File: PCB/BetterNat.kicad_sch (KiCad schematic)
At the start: 7 parts, among them J1 Conn_02x20_Odd_Even_Shielded, SW2 1825910-6, SW3 1825910-6, SW4 1825910-6, U1 KY-040

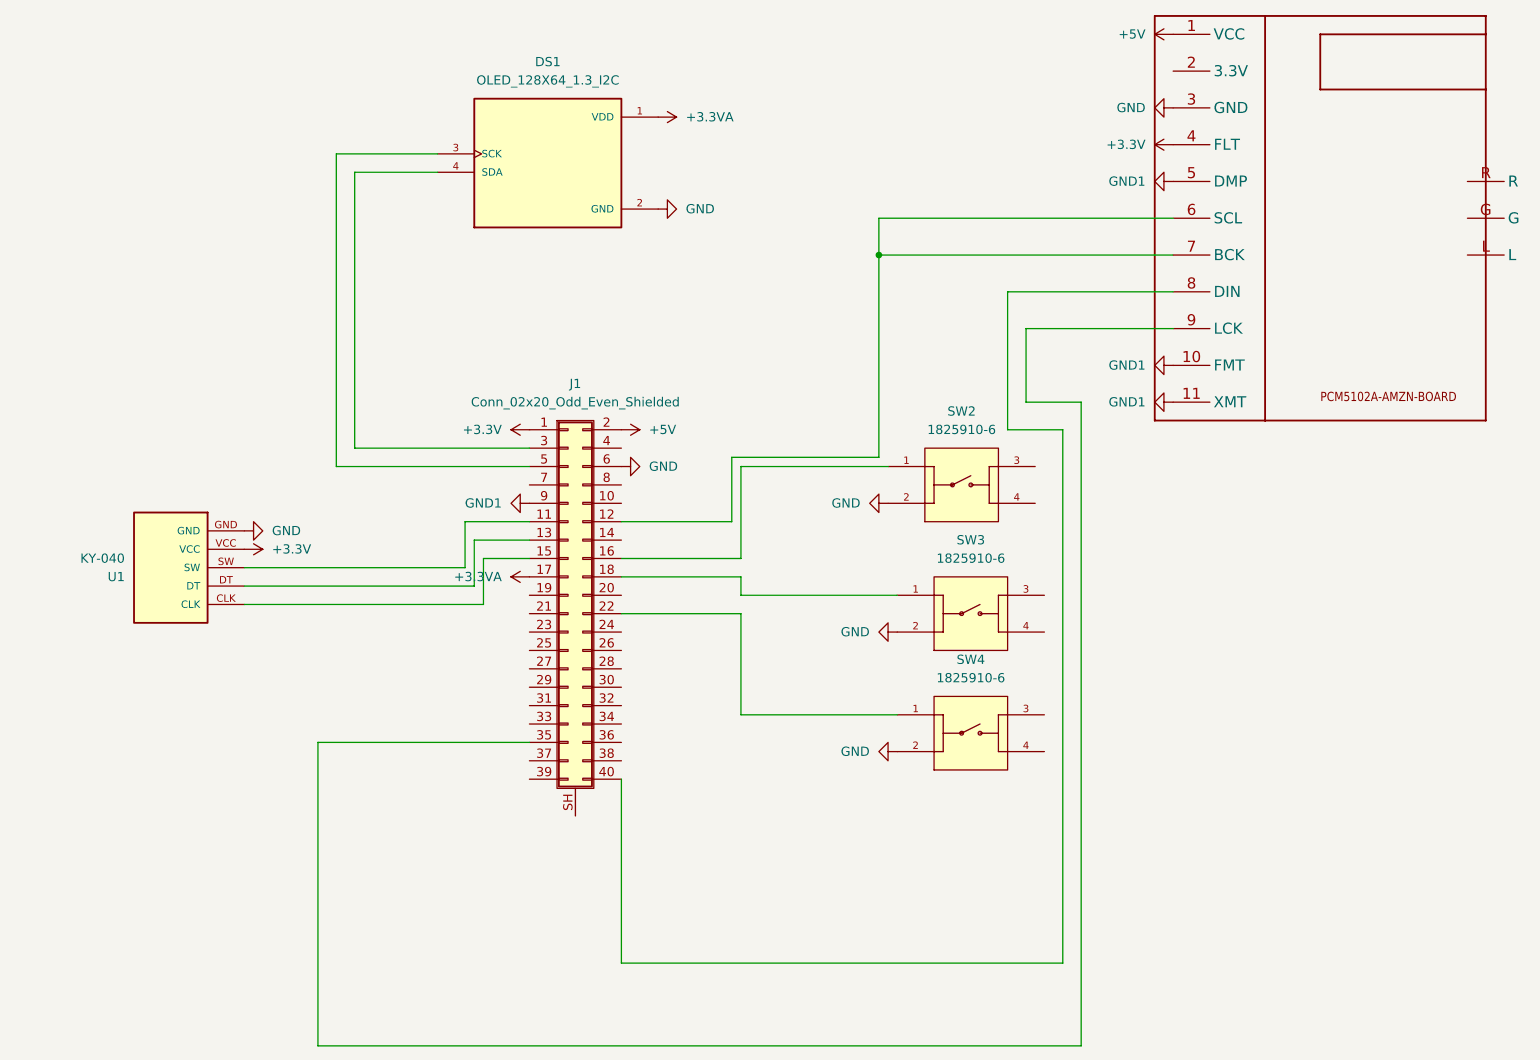
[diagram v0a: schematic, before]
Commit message: update V2
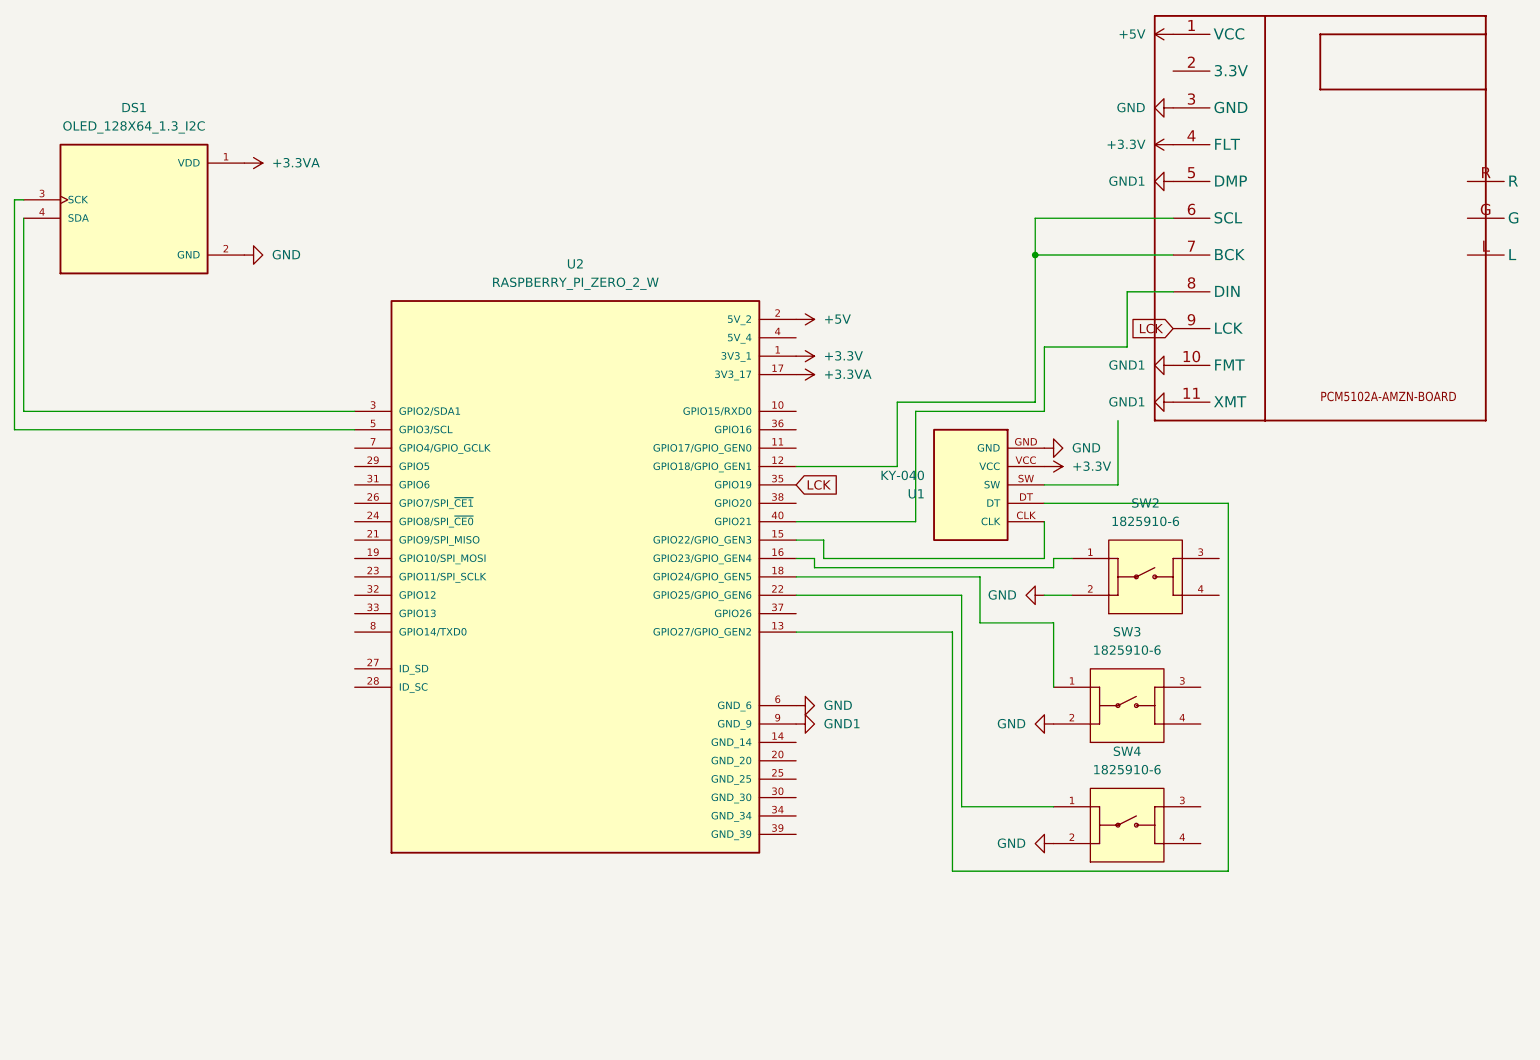
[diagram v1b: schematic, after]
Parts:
- removed J1: Conn_02x20_Odd_Even_Shielded, pin:Pin_Header_Angled_2x20_Pitch2.54mm, symbol Connector_Generic_Shielded:Conn_02x20_Odd_Even_Shielded
- added U2: RASPBERRY_PI_ZERO_2_W, 2w:MODULE_RASPBERRY_PI_ZERO_2_W3d, symbol 2w:RASPBERRY_PI_ZERO_2_W
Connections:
- net +3.3V: now also U2.1 (3V3_1)
- net +3.3VA: now also U2.17 (3V3_17)
- net +5V: now also U2.2 (5V_2)
- net GND: now also U2.6 (GND_6)
- net GND1: now also U2.9 (GND_9)
- net at SW4.1: now also U2.22 (GPIO25/GPIO_GEN6)
- net at SW3.1: now also U2.18 (GPIO24/GPIO_GEN5)
- net at DS1.3 (SCK): now also U2.5 (GPIO3/SCL)
- net at DS1.4 (SDA): now also U2.3 (GPIO2/SDA1)
- net at SW2.1: now also U2.16 (GPIO23/GPIO_GEN4)
- net at 1.6 (SCL), 1.7 (BCK): now also U2.12 (GPIO18/GPIO_GEN1)
- net at U1.DT: now also U2.13 (GPIO27/GPIO_GEN2)
- net at U1.CLK: now also U2.15 (GPIO22/GPIO_GEN3)
- net LCK: now reaches 1.9 (LCK)
- net LCK: now also U2.35 (GPIO19)
- net at 1.8 (DIN): now also U2.40 (GPIO21)
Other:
- moved on the sheet: DS1, SW2, SW3, SW4, U1
